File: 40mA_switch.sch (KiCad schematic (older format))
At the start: 4 parts, among them Q6 BC850, Q7 BC850

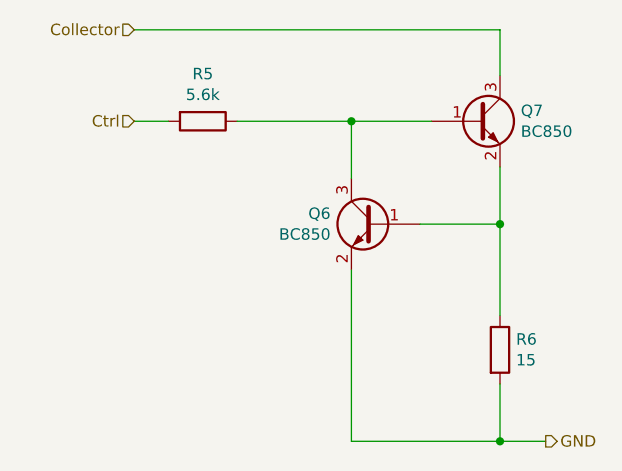
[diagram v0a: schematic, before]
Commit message: joo
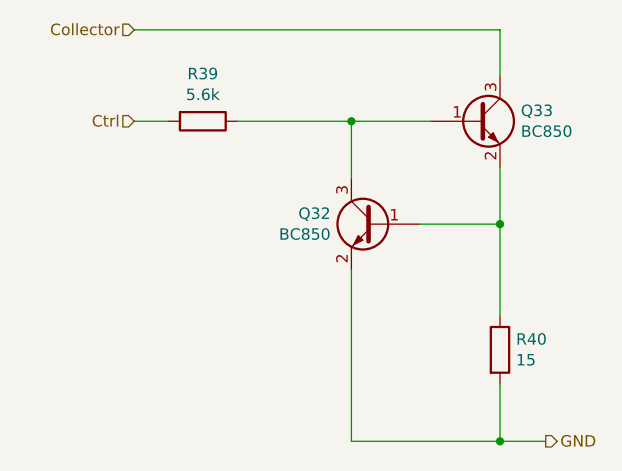
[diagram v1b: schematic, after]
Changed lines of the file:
@@
 $Descr A4 11693 8268
 encoding utf-8
-Sheet 4 22
+Sheet 17 22
 Title ""
 Date ""
@@
 AR Path="/5E309501/5E58E224/5E4F818D" Ref="R33"  Part="1"
 AR Path="/5E309501/5E58E229/5E4F818D" Ref="R39"  Part="1"
-F 0 "R5" V 1993 3900 50  0000 C CNN
+F 0 "R39" V 1993 3900 50  0000 C CNN
 F 1 "5.6k" V 2084 3900 50  0000 C CNN
 F 2 "Resistor_SMD:R_0805_2012Metric" V 2130 3900 50  0001 C CNN
@@
 AR Path="/5E309501/5E58E224/5E4F8BF8" Ref="Q31"  Part="1"
 AR Path="/5E309501/5E58E229/5E4F8BF8" Ref="Q33"  Part="1"
-F 0 "Q7" H 3591 3946 50  0000 L CNN
+F 0 "Q33" H 3591 3946 50  0000 L CNN
 F 1 "BC850" H 3591 3855 50  0000 L CNN
 F 2 "Package_TO_SOT_SMD:SOT-23" H 3600 3825 50  0001 L CIN
@@
 AR Path="/5E309501/5E58E224/5E4F9314" Ref="Q30"  Part="1"
 AR Path="/5E309501/5E58E229/5E4F9314" Ref="Q32"  Part="1"
-F 0 "Q6" H 3141 4396 50  0000 L CNN
+F 0 "Q32" H 3141 4396 50  0000 L CNN
 F 1 "BC850" H 3141 4305 50  0000 L CNN
 F 2 "Package_TO_SOT_SMD:SOT-23" H 3150 4275 50  0001 L CIN
@@
 AR Path="/5E309501/5E58E224/5E4FA760" Ref="R38"  Part="1"
 AR Path="/5E309501/5E58E229/5E4FA760" Ref="R40"  Part="1"
-F 0 "R6" H 3570 4946 50  0000 L CNN
+F 0 "R40" H 3570 4946 50  0000 L CNN
 F 1 "15" H 3570 4855 50  0000 L CNN
 F 2 "Resistor_SMD:R_0805_2012Metric" V 3430 4900 50  0001 C CNN

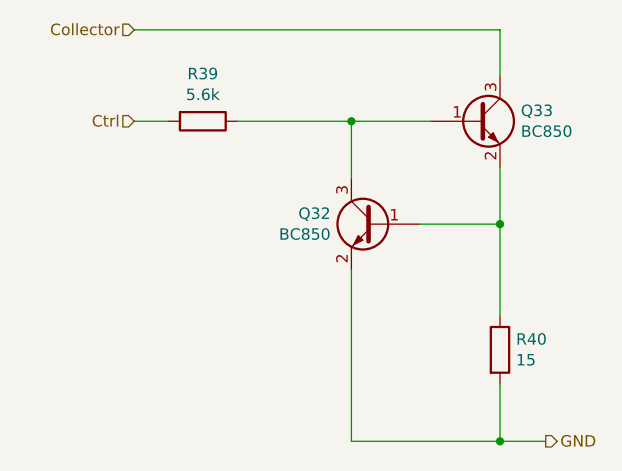
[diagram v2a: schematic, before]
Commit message: joo
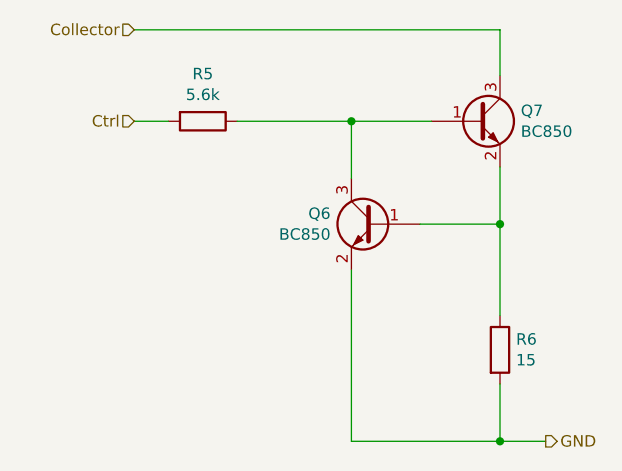
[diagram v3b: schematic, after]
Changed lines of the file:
@@
 AR Path="/5E309501/5E58E224/5E4F818D" Ref="R33"  Part="1"
 AR Path="/5E309501/5E58E229/5E4F818D" Ref="R39"  Part="1"
-F 0 "R39" V 1993 3900 50  0000 C CNN
+F 0 "R5" V 1993 3900 50  0000 C CNN
 F 1 "5.6k" V 2084 3900 50  0000 C CNN
 F 2 "Resistor_SMD:R_0805_2012Metric" V 2130 3900 50  0001 C CNN
@@
 AR Path="/5E309501/5E58E224/5E4F8BF8" Ref="Q31"  Part="1"
 AR Path="/5E309501/5E58E229/5E4F8BF8" Ref="Q33"  Part="1"
-F 0 "Q33" H 3591 3946 50  0000 L CNN
+F 0 "Q7" H 3591 3946 50  0000 L CNN
 F 1 "BC850" H 3591 3855 50  0000 L CNN
 F 2 "Package_TO_SOT_SMD:SOT-23" H 3600 3825 50  0001 L CIN
@@
 AR Path="/5E309501/5E58E224/5E4F9314" Ref="Q30"  Part="1"
 AR Path="/5E309501/5E58E229/5E4F9314" Ref="Q32"  Part="1"
-F 0 "Q32" H 3141 4396 50  0000 L CNN
+F 0 "Q6" H 3141 4396 50  0000 L CNN
 F 1 "BC850" H 3141 4305 50  0000 L CNN
 F 2 "Package_TO_SOT_SMD:SOT-23" H 3150 4275 50  0001 L CIN
@@
 AR Path="/5E309501/5E58E224/5E4FA760" Ref="R38"  Part="1"
 AR Path="/5E309501/5E58E229/5E4FA760" Ref="R40"  Part="1"
-F 0 "R40" H 3570 4946 50  0000 L CNN
+F 0 "R6" H 3570 4946 50  0000 L CNN
 F 1 "15" H 3570 4855 50  0000 L CNN
 F 2 "Resistor_SMD:R_0805_2012Metric" V 3430 4900 50  0001 C CNN
